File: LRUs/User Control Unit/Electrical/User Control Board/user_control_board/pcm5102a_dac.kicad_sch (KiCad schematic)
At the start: 2 parts, among them U2 PCM5102A

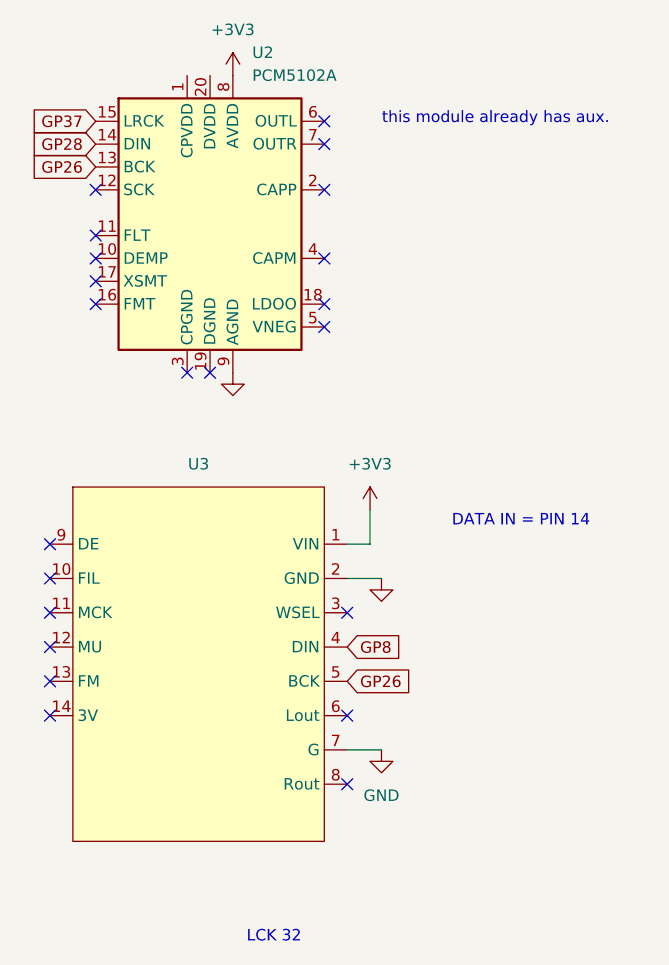
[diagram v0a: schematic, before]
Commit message: drc run
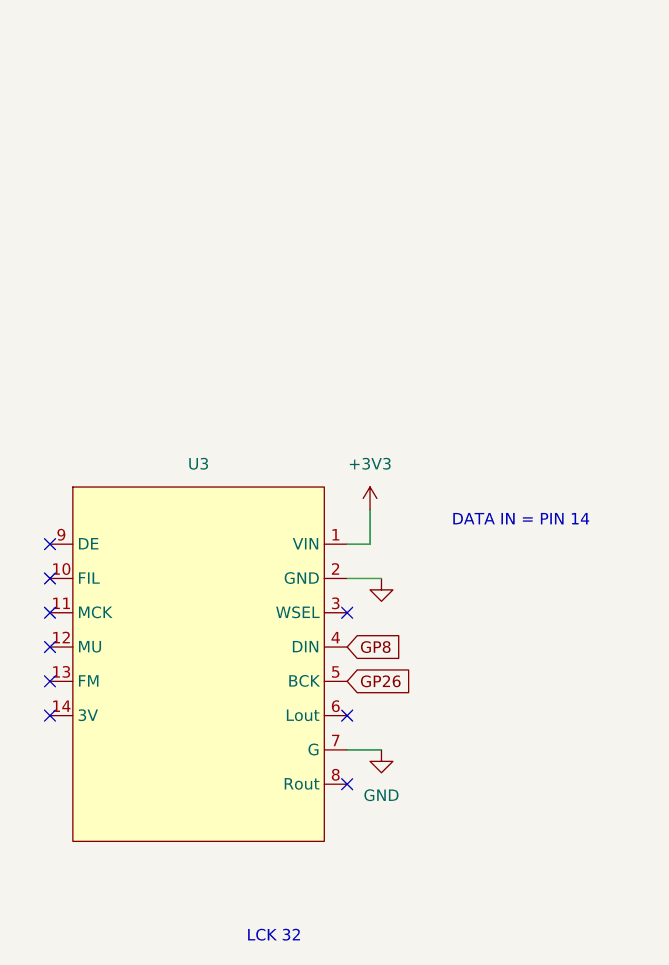
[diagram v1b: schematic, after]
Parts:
- removed U2: PCM5102A, Package_SO:TSSOP-20_4.4x6.5mm_P0.65mm, symbol Audio:PCM5102A
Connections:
- no-connect marks 22 -> 9
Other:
- note removed: "this module already has aux."
